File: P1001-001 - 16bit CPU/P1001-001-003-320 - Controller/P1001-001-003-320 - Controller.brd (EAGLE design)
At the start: 200 x 152 mm, 136 parts, among them IC1 74LS138D, IC10 74ALS00D, IC21 74LS138D, IC22 74LS138D, IC23 74LS138D, IC27 MEGA8535-A, IC3 74LS138D, IC4 74LS138D, IC5 74LS138D, J1 22-27-2041-04

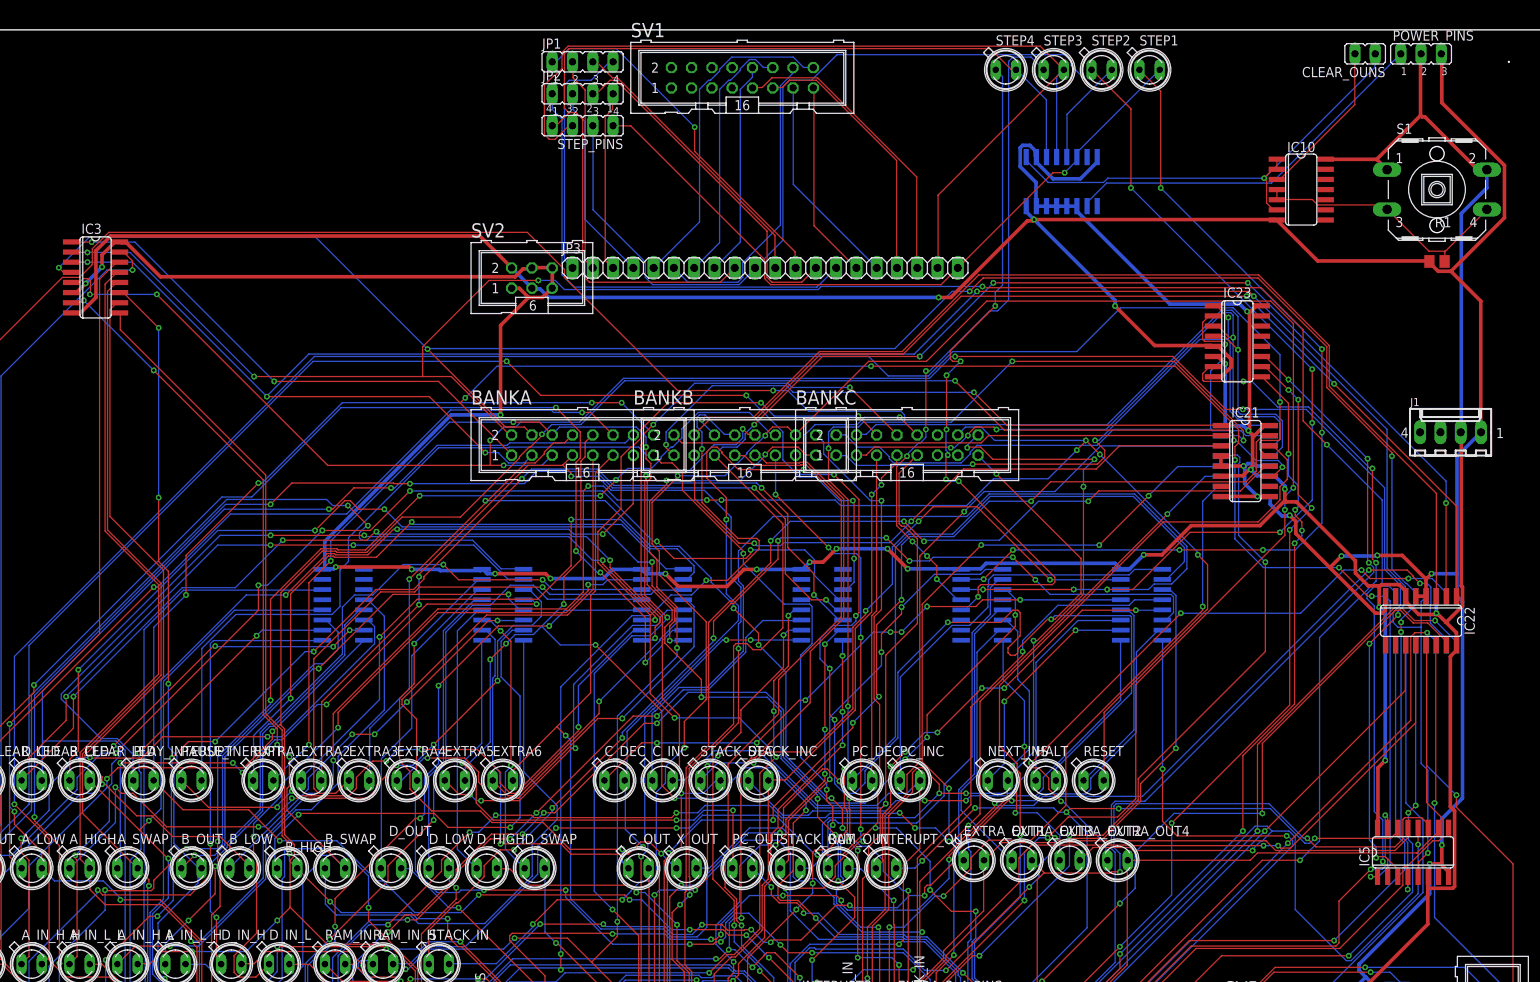
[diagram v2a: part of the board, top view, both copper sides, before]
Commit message: Finished All Boards
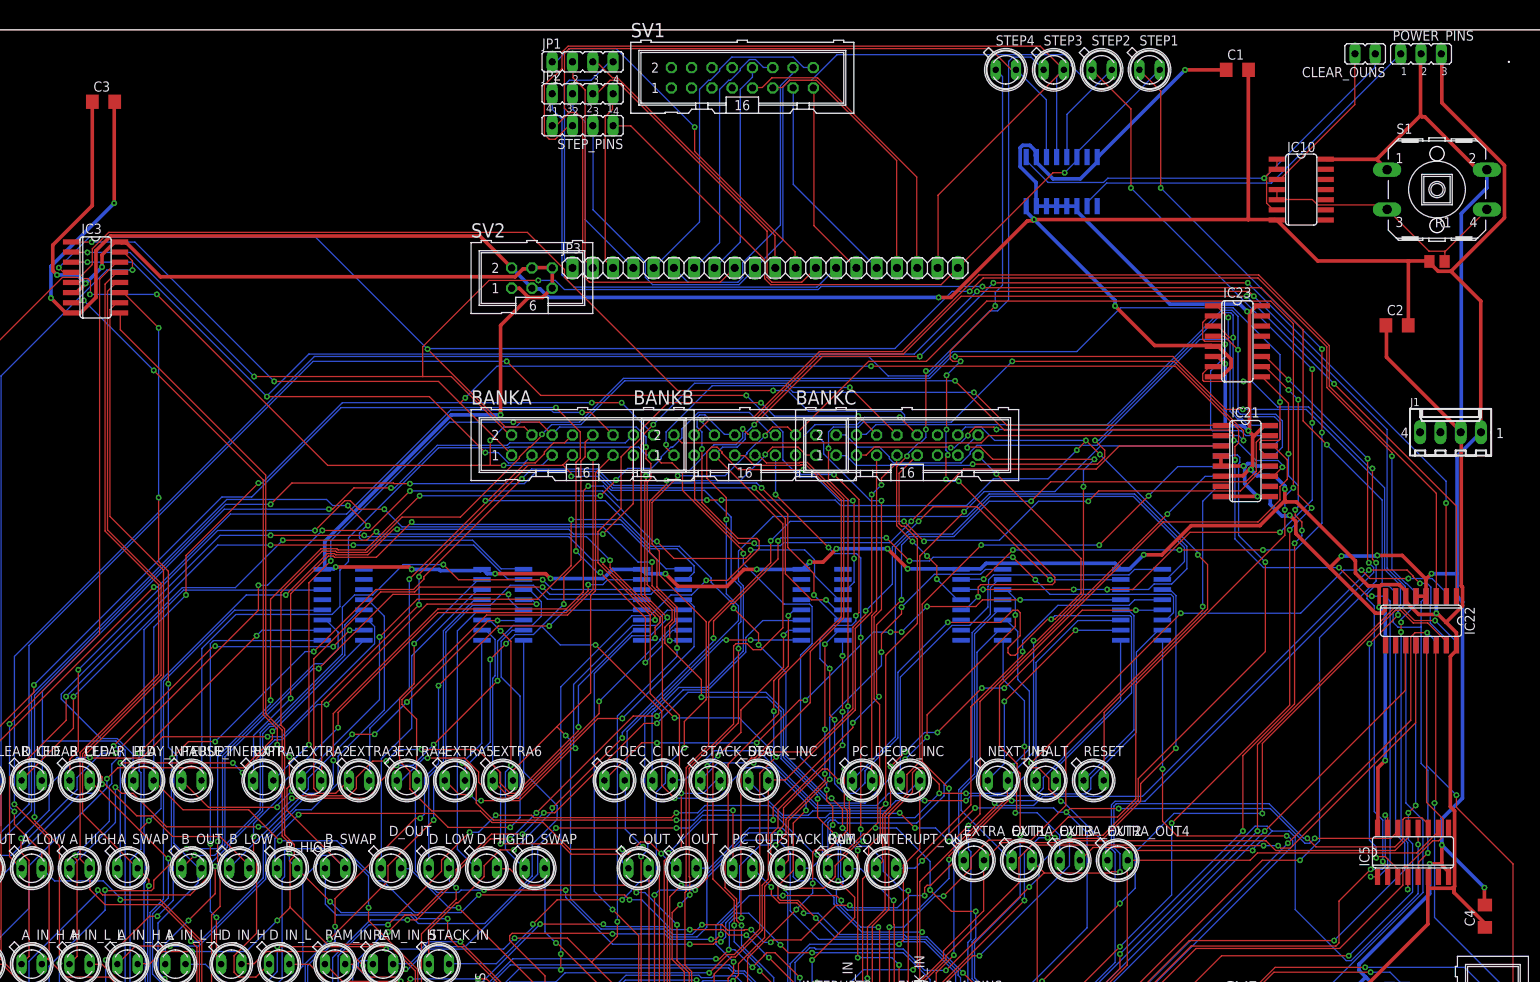
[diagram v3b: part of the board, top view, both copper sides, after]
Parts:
- added C1, C2, C3, C4: 1uF, rcl:C1206
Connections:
- net GND: now also C1.2, C2.2, C3.2, C4.2
- net VCC: now also C1.1, C2.1, C3.1, C4.1
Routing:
- net VCC: track 630.4 -> 702.9 mm, vias 26 -> 28
- net GND: track 506.9 -> 574.6 mm, vias 16 -> 19
